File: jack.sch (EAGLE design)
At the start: 29 parts, among them IC1 NUF2221W1T2G, IC2 ATSAMD21G18, IC3 LDO, SW1 SPST, X1 TSX-3225 24.0000MF10Z-C3

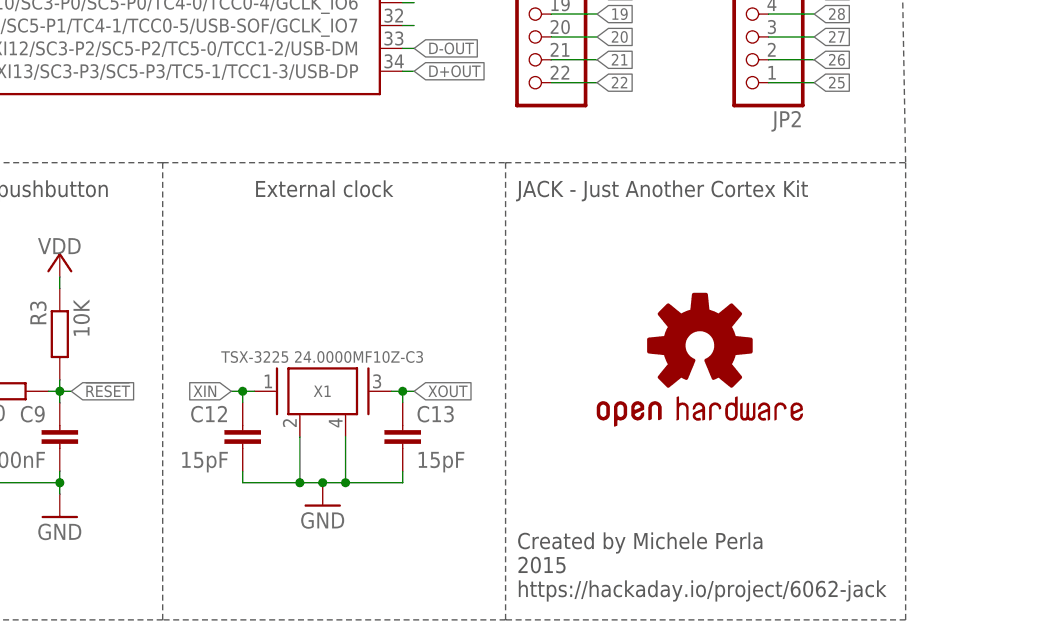
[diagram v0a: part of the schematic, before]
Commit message: Minor changes
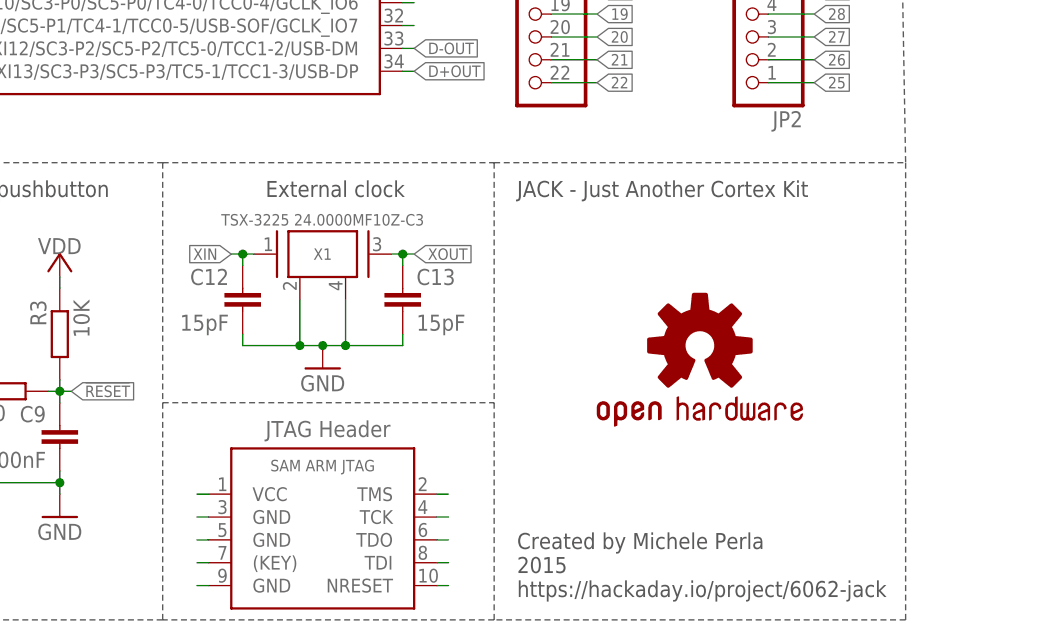
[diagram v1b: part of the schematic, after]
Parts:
- added JP3: SAM_ARM_JTAG, jack:SAM_ARM_JTAG
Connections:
- new net N$1: JP3.VCC
- new net N$10: JP3.TCK
- new net N$11: JP3.TMS
- new net N$2: JP3.GND@1
- new net N$4: JP3.GND@2
- new net N$5: JP3.(KEY)
- new net N$6: JP3.GND@3
- new net N$7: JP3.NRESET
- new net N$8: JP3.TDI
- new net N$9: JP3.TDO
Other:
- note added: "JTAG Header"
- moved on the sheet: C12, C13, X1
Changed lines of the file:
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@@
 <part name="LOGO1" library="SparkFun-Aesthetics" deviceset="OSHW-LOGO" device="L"/>
 <part name="JP2" library="pinhead" deviceset="PINHD-1X22" device=""/>
+<part name="JP3" library="jack" deviceset="SAM_ARM_JTAG" device=""/>
 </parts>
 <sheets>
@@
 <wire x1="146.05" y1="16.51" x2="147.32" y2="-54.61" width="0.1524" layer="97" style="longdash"/>
 <wire x1="147.32" y1="-54.61" x2="147.32" y2="-105.41" width="0.1524" layer="97" style="longdash"/>
-<wire x1="147.32" y1="-105.41" x2="102.87" y2="-105.41" width="0.1524" layer="97" style="longdash"/>
-<wire x1="102.87" y1="-105.41" x2="64.77" y2="-105.41" width="0.1524" layer="97" style="longdash"/>
+<wire x1="147.32" y1="-105.41" x2="101.6" y2="-105.41" width="0.1524" layer="97" style="longdash"/>
+<wire x1="101.6" y1="-105.41" x2="64.77" y2="-105.41" width="0.1524" layer="97" style="longdash"/>
 <wire x1="64.77" y1="-105.41" x2="34.29" y2="-105.41" width="0.1524" layer="97" style="longdash"/>
 <wire x1="34.29" y1="-105.41" x2="-41.91" y2="-105.41" width="0.1524" layer="97" style="longdash"/>
@@
 <text x="-17.78" y="-58.42" size="1.778" layer="97">Digital power and filter</text>
 <text x="39.37" y="-58.42" size="1.778" layer="97">Reset pushbutton</text>
-<text x="74.93" y="-58.42" size="1.778" layer="97">External clock</text>
+<text x="76.2" y="-58.42" size="1.778" layer="97">External clock</text>
 <text x="111.76" y="12.7" size="1.778" layer="97">ATSAMD21 Breakout</text>
 <wire x1="-105.41" y1="-74.93" x2="-105.41" y2="-31.75" width="0.1524" layer="97" style="longdash"/>
@@
 <wire x1="-41.91" y1="-54.61" x2="34.29" y2="-54.61" width="0.1524" layer="97" style="shortdash"/>
 <wire x1="34.29" y1="-54.61" x2="64.77" y2="-54.61" width="0.1524" layer="97" style="shortdash"/>
-<wire x1="64.77" y1="-54.61" x2="102.87" y2="-54.61" width="0.1524" layer="97" style="shortdash"/>
-<wire x1="102.87" y1="-54.61" x2="147.32" y2="-54.61" width="0.1524" layer="97" style="shortdash"/>
+<wire x1="64.77" y1="-54.61" x2="101.6" y2="-54.61" width="0.1524" layer="97" style="shortdash"/>
+<wire x1="101.6" y1="-54.61" x2="147.32" y2="-54.61" width="0.1524" layer="97" style="shortdash"/>
 <wire x1="34.29" y1="-54.61" x2="34.29" y2="-105.41" width="0.1524" layer="97" style="shortdash"/>
-<wire x1="64.77" y1="-54.61" x2="64.77" y2="-105.41" width="0.1524" layer="97" style="shortdash"/>
-<wire x1="102.87" y1="-54.61" x2="102.87" y2="-105.41" width="0.1524" layer="97" style="shortdash"/>
+<wire x1="64.77" y1="-54.61" x2="64.77" y2="-81.28" width="0.1524" layer="97" style="shortdash"/>
+<wire x1="64.77" y1="-81.28" x2="64.77" y2="-105.41" width="0.1524" layer="97" style="shortdash"/>
+<wire x1="101.6" y1="-54.61" x2="101.6" y2="-81.28" width="0.1524" layer="97" style="shortdash"/>
 <text x="104.14" y="-102.87" size="1.778" layer="97">Created by Michele Perla
 2015
 https://hackaday.io/project/6062-jack</text>
 <text x="104.14" y="-58.42" size="1.778" layer="97">JACK - Just Another Cortex Kit</text>
+<text x="76.2" y="-85.09" size="1.778" layer="95">JTAG Header</text>
+<wire x1="101.6" y1="-81.28" x2="101.6" y2="-105.41" width="0.1524" layer="97" style="shortdash"/>
+<wire x1="64.77" y1="-81.28" x2="101.6" y2="-81.28" width="0.1524" layer="97" style="shortdash"/>
 </plain>
 <instances>
@@
 <instance part="C10" gate="G$1" x="-90.17" y="-57.15" rot="MR0"/>
 <instance part="C11" gate="G$1" x="-57.15" y="-57.15"/>
-<instance part="X1" gate="G$1" x="82.55" y="-80.01"/>
-<instance part="C12" gate="G$1" x="73.66" y="-83.82" rot="MR0"/>
-<instance part="C13" gate="G$1" x="91.44" y="-83.82"/>
-<instance part="GND9" gate="G$1" x="82.55" y="-90.17"/>
+<instance part="X1" gate="G$1" x="82.55" y="-64.77"/>
+<instance part="C12" gate="G$1" x="73.66" y="-68.58" rot="MR0"/>
+<instance part="C13" gate="G$1" x="91.44" y="-68.58"/>
+<instance part="GND9" gate="G$1" x="82.55" y="-74.93"/>
 <instance part="D1" gate="G$1" x="-90.17" y="-46.99" rot="R270"/>
 <instance part="D2" gate="G$1" x="-97.79" y="-46.99" rot="R270"/>
@@
 <instance part="LOGO1" gate="G$1" x="124.46" y="-74.93"/>
 <instance part="JP2" gate="A" x="129.54" y="-20.32" rot="R180"/>
+<instance part="JP3" gate="G$1" x="82.55" y="-91.44"/>
 </instances>
 <busses>
@@
 <segment>
 <pinref part="C12" gate="G$1" pin="2"/>
-<wire x1="73.66" y1="-88.9" x2="73.66" y2="-90.17" width="0.1524" layer="91"/>
-<wire x1="73.66" y1="-90.17" x2="80.01" y2="-90.17" width="0.1524" layer="91"/>
+<wire x1="73.66" y1="-73.66" x2="73.66" y2="-74.93" width="0.1524" layer="91"/>
+<wire x1="73.66" y1="-74.93" x2="80.01" y2="-74.93" width="0.1524" layer="91"/>
 <pinref part="C13" gate="G$1" pin="2"/>
-<wire x1="80.01" y1="-90.17" x2="82.55" y2="-90.17" width="0.1524" layer="91"/>
-<wire x1="82.55" y1="-90.17" x2="85.09" y2="-90.17" width="0.1524" layer="91"/>
-<wire x1="85.09" y1="-90.17" x2="91.44" y2="-90.17" width="0.1524" layer="91"/>
-<wire x1="91.44" y1="-90.17" x2="91.44" y2="-88.9" width="0.1524" layer="91"/>
+<wire x1="80.01" y1="-74.93" x2="82.55" y2="-74.93" width="0.1524" layer="91"/>
+<wire x1="82.55" y1="-74.93" x2="85.09" y2="-74.93" width="0.1524" layer="91"/>
+<wire x1="85.09" y1="-74.93" x2="91.44" y2="-74.93" width="0.1524" layer="91"/>
+<wire x1="91.44" y1="-74.93" x2="91.44" y2="-73.66" width="0.1524" layer="91"/>
 <pinref part="X1" gate="G$1" pin="GND@1"/>
-<wire x1="80.01" y1="-85.09" x2="80.01" y2="-90.17" width="0.1524" layer="91"/>
+<wire x1="80.01" y1="-69.85" x2="80.01" y2="-74.93" width="0.1524" layer="91"/>
 <pinref part="X1" gate="G$1" pin="GND@2"/>
-<wire x1="85.09" y1="-85.09" x2="85.09" y2="-90.17" width="0.1524" layer="91"/>
-<junction x="80.01" y="-90.17"/>
-<junction x="85.09" y="-90.17"/>
-<junction x="82.55" y="-90.17"/>
+<wire x1="85.09" y1="-69.85" x2="85.09" y2="-74.93" width="0.1524" layer="91"/>
+<junction x="80.01" y="-74.93"/>
+<junction x="85.09" y="-74.93"/>
+<junction x="82.55" y="-74.93"/>
 <pinref part="GND9" gate="G$1" pin="GND"/>
 </segment>
@@
 <segment>
 <pinref part="X1" gate="G$1" pin="P$1"/>
-<wire x1="74.93" y1="-80.01" x2="73.66" y2="-80.01" width="0.1524" layer="91"/>
+<wire x1="74.93" y1="-64.77" x2="73.66" y2="-64.77" width="0.1524" layer="91"/>
 <pinref part="C12" gate="G$1" pin="1"/>
-<wire x1="73.66" y1="-80.01" x2="73.66" y2="-81.28" width="0.1524" layer="91"/>
-<junction x="73.66" y="-80.01"/>
-<wire x1="73.66" y1="-80.01" x2="72.39" y2="-80.01" width="0.1524" layer="91"/>
-<label x="72.39" y="-80.01" size="1.27" layer="95" rot="R180" xref="yes"/>
+<wire x1="73.66" y1="-64.77" x2="73.66" y2="-66.04" width="0.1524" layer="91"/>
+<junction x="73.66" y="-64.77"/>
+<wire x1="73.66" y1="-64.77" x2="72.39" y2="-64.77" width="0.1524" layer="91"/>
+<label x="72.39" y="-64.77" size="1.27" layer="95" rot="R180" xref="yes"/>
 </segment>
 </net>
@@
 <segment>
 <pinref part="X1" gate="G$1" pin="P$3"/>
-<wire x1="90.17" y1="-80.01" x2="91.44" y2="-80.01" width="0.1524" layer="91"/>
+<wire x1="90.17" y1="-64.77" x2="91.44" y2="-64.77" width="0.1524" layer="91"/>
 <pinref part="C13" gate="G$1" pin="1"/>
-<wire x1="91.44" y1="-80.01" x2="91.44" y2="-81.28" width="0.1524" layer="91"/>
-<junction x="91.44" y="-80.01"/>
-<wire x1="91.44" y1="-80.01" x2="92.71" y2="-80.01" width="0.1524" layer="91"/>
-<label x="92.71" y="-80.01" size="1.27" layer="95" xref="yes"/>
+<wire x1="91.44" y1="-64.77" x2="91.44" y2="-66.04" width="0.1524" layer="91"/>
+<junction x="91.44" y="-64.77"/>
+<wire x1="91.44" y1="-64.77" x2="92.71" y2="-64.77" width="0.1524" layer="91"/>
+<label x="92.71" y="-64.77" size="1.27" layer="95" xref="yes"/>
 </segment>
 </net>
@@
 </segment>
 </net>
+<net name="N$1" class="0">
+<segment>
+<pinref part="JP3" gate="G$1" pin="VCC"/>
+<wire x1="69.85" y1="-91.44" x2="68.58" y2="-91.44" width="0.1524" layer="91"/>
+</segment>
+</net>
+<net name="N$2" class="0">
+<segment>
+<pinref part="JP3" gate="G$1" pin="GND@1"/>
+<wire x1="69.85" y1="-93.98" x2="68.58" y2="-93.98" width="0.1524" layer="91"/>
+</segment>
+</net>
+<net name="N$4" class="0">
+<segment>
+<pinref part="JP3" gate="G$1" pin="GND@2"/>
+<wire x1="69.85" y1="-96.52" x2="68.58" y2="-96.52" width="0.1524" layer="91"/>
+</segment>
+</net>
+<net name="N$5" class="0">
+<segment>
+<pinref part="JP3" gate="G$1" pin="(KEY)"/>
+<wire x1="69.85" y1="-99.06" x2="68.58" y2="-99.06" width="0.1524" layer="91"/>
+</segment>
+</net>
+<net name="N$6" class="0">
+<segment>
+<pinref part="JP3" gate="G$1" pin="GND@3"/>
+<wire x1="69.85" y1="-101.6" x2="68.58" y2="-101.6" width="0.1524" layer="91"/>
+</segment>
+</net>
+<net name="N$7" class="0">
+<segment>
+<pinref part="JP3" gate="G$1" pin="NRESET"/>
+<wire x1="95.25" y1="-101.6" x2="96.52" y2="-101.6" width="0.1524" layer="91"/>
+</segment>
+</net>
+<net name="N$8" class="0">
+<segment>
+<pinref part="JP3" gate="G$1" pin="TDI"/>
+<wire x1="95.25" y1="-99.06" x2="96.52" y2="-99.06" width="0.1524" layer="91"/>
+</segment>
+</net>
+<net name="N$9" class="0">
+<segment>
+<pinref part="JP3" gate="G$1" pin="TDO"/>
+<wire x1="95.25" y1="-96.52" x2="96.52" y2="-96.52" width="0.1524" layer="91"/>
+</segment>
+</net>
+<net name="N$10" class="0">
+<segment>
+<pinref part="JP3" gate="G$1" pin="TCK"/>
+<wire x1="95.25" y1="-93.98" x2="96.52" y2="-93.98" width="0.1524" layer="91"/>
+</segment>
+</net>
+<net name="N$11" class="0">
+<segment>
+<pinref part="JP3" gate="G$1" pin="TMS"/>
+<wire x1="95.25" y1="-91.44" x2="96.52" y2="-91.44" width="0.1524" layer="91"/>
+</segment>
+</net>
